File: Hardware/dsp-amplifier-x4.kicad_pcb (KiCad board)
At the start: 2 copper layers, 104 parts, among them J1 Raspberry_Pi_2_3, J2 USB_B, J3 USBi, Q1 STD2805, U1 ADAU1452, U2 24LC1025, U3 SI53365, U5 TPS54308, U6 TPS54308, U7 AMS1117-3.3, U8 USBLC6-2SC6, U9 PCM2707, Y1 12 MHz

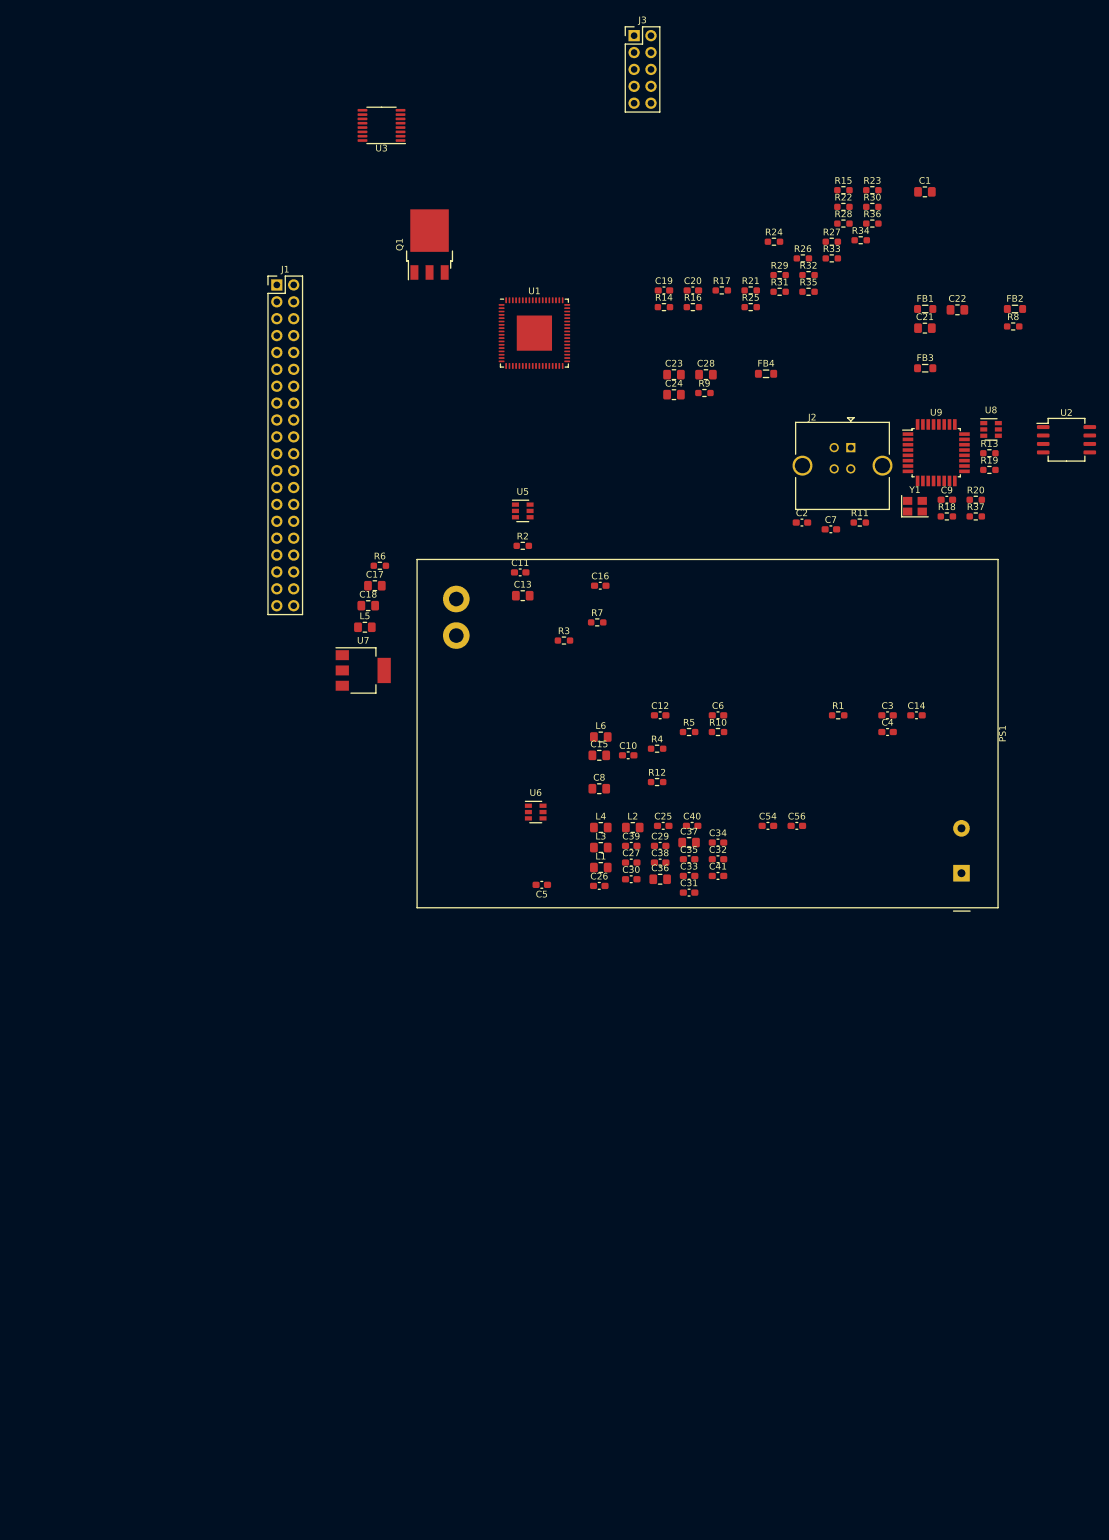
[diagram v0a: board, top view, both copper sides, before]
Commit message: various fixes
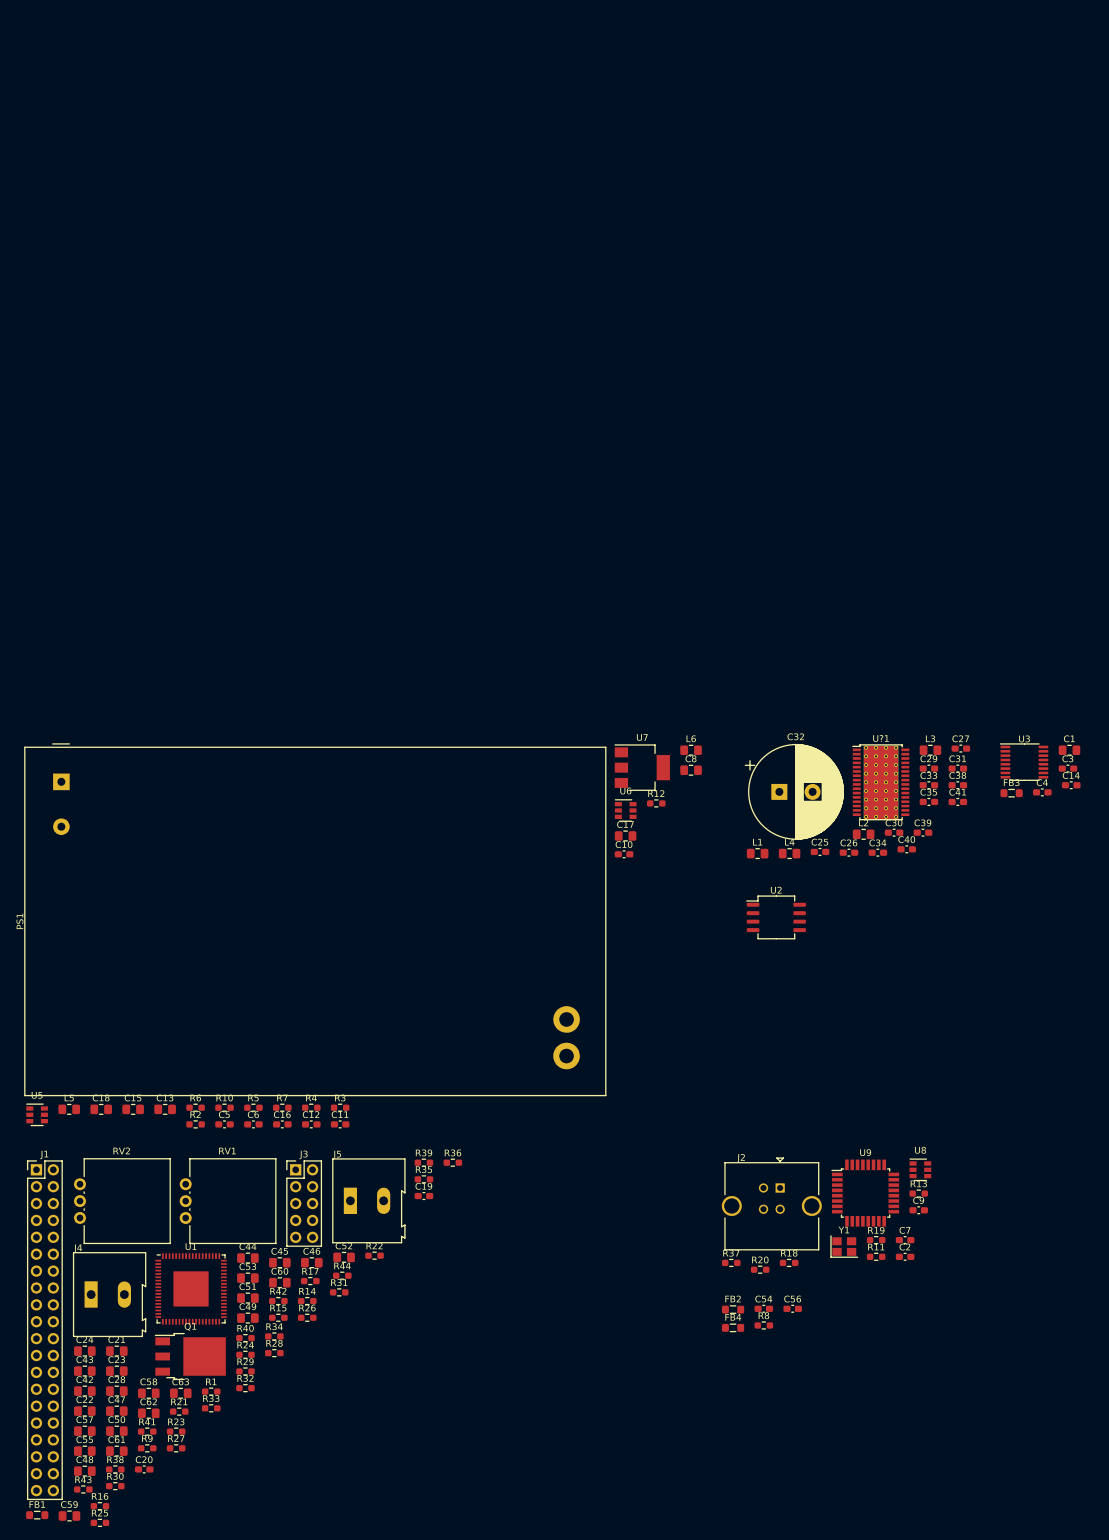
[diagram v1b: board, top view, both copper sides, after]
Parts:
- removed C36, C37: 4.7u, Capacitor_SMD:C_0805_2012Metric_Pad1.18x1.45mm_HandSolder
- added C42: 10n, Capacitor_SMD:C_0805_2012Metric_Pad1.18x1.45mm_HandSolder, F.Cu at (54.4, 138.2)
- added C43: 10n, Capacitor_SMD:C_0805_2012Metric_Pad1.18x1.45mm_HandSolder, F.Cu at (54.4, 135.2)
- added C44: 10n, Capacitor_SMD:C_0805_2012Metric_Pad1.18x1.45mm_HandSolder, F.Cu at (78.9, 118.2)
- added C45: 100n, Capacitor_SMD:C_0805_2012Metric_Pad1.18x1.45mm_HandSolder, F.Cu at (83.7, 118.8)
- added C46: 100n, Capacitor_SMD:C_0805_2012Metric_Pad1.18x1.45mm_HandSolder, F.Cu at (88.5, 118.8)
- added C47: 100n, Capacitor_SMD:C_0805_2012Metric_Pad1.18x1.45mm_HandSolder, F.Cu at (59.2, 141.2)
- added C48: 10n, Capacitor_SMD:C_0805_2012Metric_Pad1.18x1.45mm_HandSolder, F.Cu at (54.4, 150.2)
- added C49: 10n, Capacitor_SMD:C_0805_2012Metric_Pad1.18x1.45mm_HandSolder, F.Cu at (78.9, 127.2)
- added C50: 10n, Capacitor_SMD:C_0805_2012Metric_Pad1.18x1.45mm_HandSolder, F.Cu at (59.2, 144.2)
- added C51: 100n, Capacitor_SMD:C_0805_2012Metric_Pad1.18x1.45mm_HandSolder, F.Cu at (78.9, 124.2)
- added C52: 100n, Capacitor_SMD:C_0805_2012Metric_Pad1.18x1.45mm_HandSolder, F.Cu at (93.4, 118.0)
- added C53: 100n, Capacitor_SMD:C_0805_2012Metric_Pad1.18x1.45mm_HandSolder, F.Cu at (78.9, 121.2)
- added C55: 10n, Capacitor_SMD:C_0805_2012Metric_Pad1.18x1.45mm_HandSolder, F.Cu at (54.4, 147.2)
- added C57: 10n, Capacitor_SMD:C_0805_2012Metric_Pad1.18x1.45mm_HandSolder, F.Cu at (54.4, 144.2)
- added C58: 100n, Capacitor_SMD:C_0805_2012Metric_Pad1.18x1.45mm_HandSolder, F.Cu at (64.0, 138.5)
- added C59: 100n, Capacitor_SMD:C_0805_2012Metric_Pad1.18x1.45mm_HandSolder, F.Cu at (52.1, 156.9)
- added C60: 10n, Capacitor_SMD:C_0805_2012Metric_Pad1.18x1.45mm_HandSolder, F.Cu at (83.7, 121.9)
- added C61: 10n, Capacitor_SMD:C_0805_2012Metric_Pad1.18x1.45mm_HandSolder, F.Cu at (59.2, 147.2)
- added C62: 100n, Capacitor_SMD:C_0805_2012Metric_Pad1.18x1.45mm_HandSolder, F.Cu at (64.0, 141.5)
- added C63: 100n, Capacitor_SMD:C_0805_2012Metric_Pad1.18x1.45mm_HandSolder, F.Cu at (68.8, 138.5)
- added J4: Screw_Terminal_01x02, TerminalBlock:TerminalBlock_Altech_AK300-2_P5.00mm, F.Cu at (55.3, 123.6)
- added J5: Screw_Terminal_01x02, TerminalBlock:TerminalBlock_Altech_AK300-2_P5.00mm, F.Cu at (94.3, 109.5)
- added R38: 33, Resistor_SMD:R_0603_1608Metric_Pad0.98x0.95mm_HandSolder, F.Cu at (59.0, 149.9)
- added R39: 33, Resistor_SMD:R_0603_1608Metric_Pad0.98x0.95mm_HandSolder, F.Cu at (105.4, 103.8)
- added R40: 33, Resistor_SMD:R_0603_1608Metric_Pad0.98x0.95mm_HandSolder, F.Cu at (78.5, 130.2)
- added R41: 4.3k, Resistor_SMD:R_0603_1608Metric_Pad0.98x0.95mm_HandSolder, F.Cu at (63.8, 144.3)
- added R42: DNP, Resistor_SMD:R_0603_1608Metric_Pad0.98x0.95mm_HandSolder, F.Cu at (83.5, 124.6)
- added R43: DNP, Resistor_SMD:R_0603_1608Metric_Pad0.98x0.95mm_HandSolder, F.Cu at (54.1, 153.0)
- added R44: 4.3k, Resistor_SMD:R_0603_1608Metric_Pad0.98x0.95mm_HandSolder, F.Cu at (93.1, 120.8)
- added RV1: R_POT, Potentiometer_THT:Potentiometer_Vishay_248GJ-249GJ_Single_Vertical, F.Cu at (69.5, 112.1)
- added RV2: R_POT, Potentiometer_THT:Potentiometer_Vishay_248GJ-249GJ_Single_Vertical, F.Cu at (53.6, 112.1)
- added U?1: TAS5760MDCAR, Package_SO:HTSSOP-32-1EP_6.1x11mm_P0.65mm_EP5.2x11mm_Mask4.11x4.36mm_ThermalVias, F.Cu at (174.2, 46.6)
- C25: value 1u -> 100n
- C32: value 100n -> 470u; footprint Capacitor_SMD:C_0603_1608Metric_Pad1.08x0.95mm_HandSolder -> Capacitor_THT:CP_Radial_D14.0mm_P5.00mm
- moved FB1 225.3 mm to (47.2, 156.8)
- moved R30 223.6 mm to (59.0, 152.5)
- moved R23 214.1 mm to (68.1, 144.3)
- moved C22 211.4 mm to (54.4, 141.2)
- moved R25 207.4 mm to (56.6, 158.0)
- moved R27 206.6 mm to (68.1, 146.8)
- moved R16 201.2 mm to (56.6, 155.5)
- moved R33 196.6 mm to (73.4, 140.8)
- moved C21 196.1 mm to (59.2, 132.1)
- moved C20 195.6 mm to (63.3, 149.9)
- moved R28 190.3 mm to (82.9, 132.4)
- moved R15 189.7 mm to (83.5, 127.1)
- moved R21 189.3 mm to (68.6, 141.2)
- moved R32 187.7 mm to (78.5, 137.7)
- moved R34 187.0 mm to (82.9, 129.9)
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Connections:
- C25 pad 1: +3V3 -> +24V
- C26 pad 2: (no net) -> Net-(C26-Pad2)
- C27 pad 2: (no net) -> Net-(C27-Pad2)
- C29 pad 2: (no net) -> Net-(C29-Pad2)
- C30 pad 1: (no net) -> Net-(C30-Pad1)
- C33 pad 2: (no net) -> Net-(C33-Pad2)
- C34 pad 2: (no net) -> Net-(C34-Pad2)
- Q1 pad 1: Net-(Q1-Pad1) -> /VDRIVE
- R1 pad 2: Net-(Q1-Pad1) -> /VDRIVE
- R22 pad 1: (no net) -> /AMP1_LRCLK
- R23 pad 1: (no net) -> /AMP1_BCLK
- R24 pad 1: (no net) -> /AMP1_SDIN
- U1 pad 26: (no net) -> /AMP1_NSPK_SD
- U1 pad 27: (no net) -> /AMP1_SPK_SLEEP
- U1 pad 3: (no net) -> /VDRIVE
- U1 pad 42: (no net) -> Net-(R38-Pad2)
- U1 pad 43: (no net) -> Net-(R39-Pad2)
- U1 pad 44: (no net) -> Net-(R40-Pad2)
- U1 pad 66: (no net) -> /EXT_O_LRCLK
- U1 pad 8: (no net) -> /VPOT0
- U1 pad 9: (no net) -> /VPOT1
- U3 pad 16: (no net) -> /AMP1_CLOCK
